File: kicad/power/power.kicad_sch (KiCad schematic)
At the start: 8 parts, among them J1 Power IN, J2 OLED_in, J3 SW_Power, J4 OLED_out, J5 Power OUT

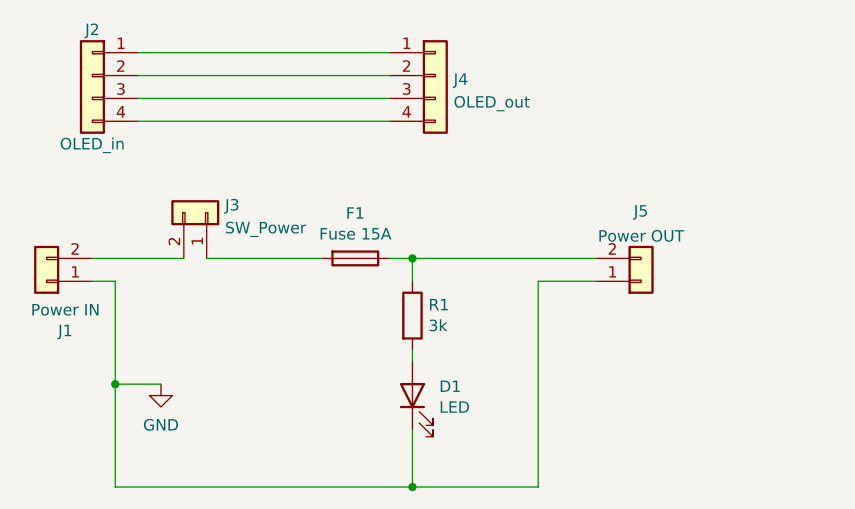
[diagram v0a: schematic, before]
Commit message: fix
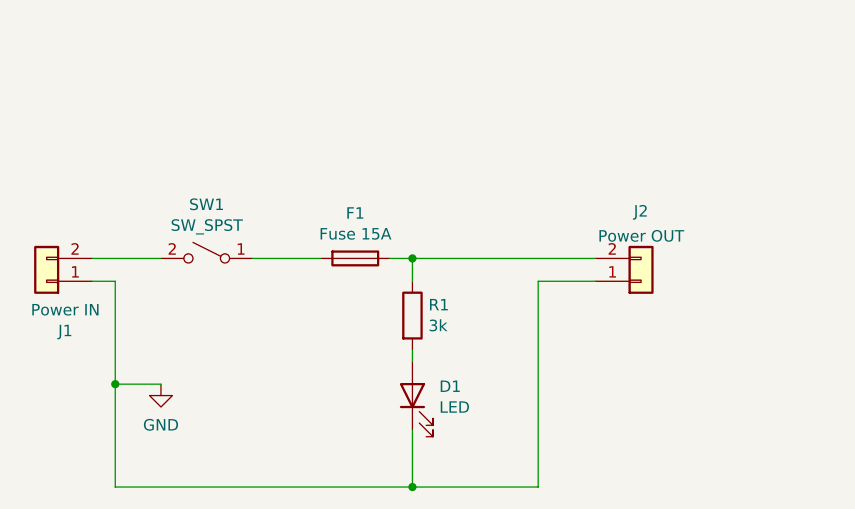
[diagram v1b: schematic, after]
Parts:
- removed J2: OLED_in, 0.main.robot:JSTS4B-ZRLFSN, symbol Connector_Generic:Conn_01x04
- removed J3: SW_Power, Connector_JST:JST_VH_B2PS-VH_1x02_P3.96mm_Horizontal, symbol Connector_Generic:Conn_01x02
- removed J4: OLED_out, Connector_PinSocket_2.54mm:PinSocket_1x04_P2.54mm_Vertical, symbol Connector_Generic:Conn_01x04
- added SW1: SW_SPST, 0.main.robot:SW_SPST_POWER, symbol Switch:SW_SPST
- renumbered J5 to J2
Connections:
- net at F1.2: now also SW1.1 (A)
- net at J1.2 (Pin_2): now also SW1.2 (B)
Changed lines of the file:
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@@
   (junction (at 162.56 83.82) (diameter 0) (color 0 0 0 0)
   )
-  (wire (pts (xy 162.56 83.82) (xy 162.56 86.36))
+  (wire (pts (xy 144.78 83.82) (xy 152.4 83.82))
     (stroke (width 0) (type default) (color 0 0 0 0))
   )
-  (wire (pts (xy 139.7 83.82) (xy 152.4 83.82))
+  (wire (pts (xy 162.56 83.82) (xy 162.56 86.36))
     (stroke (width 0) (type default) (color 0 0 0 0))
   )
@@
     (stroke (width 0) (type default) (color 0 0 0 0))
   )
-  (wire (pts (xy 127 83.82) (xy 137.16 83.82))
-    (stroke (width 0) (type default) (color 0 0 0 0))
-  )
   (wire (pts (xy 162.56 109.22) (xy 176.53 109.22))
     (stroke (width 0) (type default) (color 0 0 0 0))
   )
-  (wire (pts (xy 132.08 68.58) (xy 160.02 68.58))
+  (wire (pts (xy 127 86.36) (xy 129.54 86.36))
     (stroke (width 0) (type default) (color 0 0 0 0))
   )
-  (wire (pts (xy 127 86.36) (xy 129.54 86.36))
+  (wire (pts (xy 127 83.82) (xy 134.62 83.82))
     (stroke (width 0) (type default) (color 0 0 0 0))
   )
@@
     (stroke (width 0) (type default) (color 0 0 0 0))
   )
-  (wire (pts (xy 132.08 66.04) (xy 160.02 66.04))
-    (stroke (width 0) (type default) (color 0 0 0 0))
-  )
   (wire (pts (xy 162.56 83.82) (xy 182.88 83.82))
     (stroke (width 0) (type default) (color 0 0 0 0))
@@
     (stroke (width 0) (type default) (color 0 0 0 0))
   )
-  (wire (pts (xy 132.08 63.5) (xy 160.02 63.5))
-    (stroke (width 0) (type default) (color 0 0 0 0))
-  )
   (wire (pts (xy 176.53 86.36) (xy 182.88 86.36))
-    (stroke (width 0) (type default) (color 0 0 0 0))
-  )
-  (wire (pts (xy 132.08 60.96) (xy 160.02 60.96))
     (stroke (width 0) (type default) (color 0 0 0 0))
   )
@@
     (pin "2")
   )
-  (symbol (lib_id "Connector_Generic:Conn_01x04") (at 165.1 63.5 0) (unit 1)
-    (in_bom yes) (on_board yes) (fields_autoplaced)
-    (property "Reference" "J4" (id 0) (at 167.132 63.9353 0)
-      (effects (font (size 1.27 1.27)) (justify left))
-    )
-    (property "Value" "OLED_out" (id 1) (at 167.132 66.4722 0)
-      (effects (font (size 1.27 1.27)) (justify left))
-    )
-    (property "Footprint" "Connector_PinSocket_2.54mm:PinSocket_1x04_P2.54mm_Vertical" (id 2) (at 165.1 63.5 0)
-      (effects (font (size 1.27 1.27)) hide)
-    )
-    (property "Datasheet" "~" (id 3) (at 165.1 63.5 0)
-      (effects (font (size 1.27 1.27)) hide)
-    )
-    (pin "1")
-    (pin "2")
-    (pin "3")
-    (pin "4")
-  )
   (symbol (lib_id "Device:Fuse") (at 156.21 83.82 270) (unit 1)
     (in_bom yes) (on_board yes)
@@
     (pin "1")
     (pin "2")
-  )
-  (symbol (lib_id "Connector_Generic:Conn_01x02") (at 139.7 78.74 270) (mirror x) (unit 1)
-    (in_bom yes) (on_board yes) (fields_autoplaced)
-    (property "Reference" "J3" (id 0) (at 141.732 77.9053 90)
-      (effects (font (size 1.27 1.27)) (justify left))
-    )
-    (property "Value" "SW_Power" (id 1) (at 141.732 80.4422 90)
-      (effects (font (size 1.27 1.27)) (justify left))
-    )
-    (property "Footprint" "Connector_JST:JST_VH_B2PS-VH_1x02_P3.96mm_Horizontal" (id 2) (at 139.7 78.74 0)
-      (effects (font (size 1.27 1.27)) hide)
-    )
-    (property "Datasheet" "~" (id 3) (at 139.7 78.74 0)
-      (effects (font (size 1.27 1.27)) hide)
-    )
-    (pin "1")
-    (pin "2")
-  )
-  (symbol (lib_id "Connector_Generic:Conn_01x04") (at 127 63.5 0) (mirror y) (unit 1)
-    (in_bom yes) (on_board yes)
-    (property "Reference" "J2" (id 0) (at 127 58.42 0))
-    (property "Value" "OLED_in" (id 1) (at 127 71.12 0))
-    (property "Footprint" "0.main.robot:JSTS4B-ZRLFSN" (id 2) (at 127 63.5 0)
-      (effects (font (size 1.27 1.27)) hide)
-    )
-    (property "Datasheet" "~" (id 3) (at 127 63.5 0)
-      (effects (font (size 1.27 1.27)) hide)
-    )
-    (pin "1")
-    (pin "2")
-    (pin "3")
-    (pin "4")
   )
   (symbol (lib_id "Connector_Generic:Conn_01x02") (at 121.92 86.36 180) (unit 1)
@@
     (pin "2")
   )
+  (symbol (lib_id "Switch:SW_SPST") (at 139.7 83.82 0) (mirror y) (unit 1)
+    (in_bom yes) (on_board yes)
+    (property "Reference" "SW1" (id 0) (at 139.7 77.851 0))
+    (property "Value" "SW_SPST" (id 1) (at 139.7 80.1624 0))
+    (property "Footprint" "0.main.robot:SW_SPST_POWER" (id 2) (at 139.7 83.82 0)
+      (effects (font (size 1.27 1.27)) hide)
+    )
+    (property "Datasheet" "~" (id 3) (at 139.7 83.82 0)
+      (effects (font (size 1.27 1.27)) hide)
+    )
+    (pin "1")
+    (pin "2")
+  )
   (symbol (lib_id "Connector_Generic:Conn_01x02") (at 187.96 86.36 0) (mirror x) (unit 1)
     (in_bom yes) (on_board yes) (fields_autoplaced)
-    (property "Reference" "J5" (id 0) (at 187.96 78.5835 0))
+    (property "Reference" "J2" (id 0) (at 187.96 78.5835 0))
     (property "Value" "Power OUT" (id 1) (at 187.96 81.3586 0))
     (property "Footprint" "Connector_JST:JST_VH_B2PS-VH_1x02_P3.96mm_Horizontal" (id 2) (at 187.96 86.36 0)
@@
       (reference "J1") (unit 1) (value "Power IN") (footprint "0.main.robot:AMASS_XT60-M_1x02_P7.20mm_Vertical")
     )
-    (path "/598e9a76-0db2-44a9-a60c-d4ed24c476ce"
-      (reference "J2") (unit 1) (value "OLED_in") (footprint "0.main.robot:JSTS4B-ZRLFSN")
-    )
-    (path "/5499bae8-d48d-4f07-8f5a-e4889474cbb5"
-      (reference "J3") (unit 1) (value "SW_Power") (footprint "Connector_JST:JST_VH_B2PS-VH_1x02_P3.96mm_Horizontal")
-    )
-    (path "/10f6edf7-7273-449a-9f23-cf75ddf38fd1"
-      (reference "J4") (unit 1) (value "OLED_out") (footprint "Connector_PinSocket_2.54mm:PinSocket_1x04_P2.54mm_Vertical")
-    )
     (path "/885e45ca-60a4-45d9-b880-170c39d96ea5"
-      (reference "J5") (unit 1) (value "Power OUT") (footprint "Connector_JST:JST_VH_B2PS-VH_1x02_P3.96mm_Horizontal")
+      (reference "J2") (unit 1) (value "Power OUT") (footprint "Connector_JST:JST_VH_B2PS-VH_1x02_P3.96mm_Horizontal")
     )
     (path "/10672f86-6d1c-4735-823d-6815512456a3"
       (reference "R1") (unit 1) (value "3k") (footprint "Resistor_SMD:R_0603_1608Metric_Pad0.98x0.95mm_HandSolder")
     )
+    (path "/860b1473-4398-44af-9a5d-d556293557fc"
+      (reference "SW1") (unit 1) (value "SW_SPST") (footprint "0.main.robot:SW_SPST_POWER")
+    )
   )

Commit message: fix: power
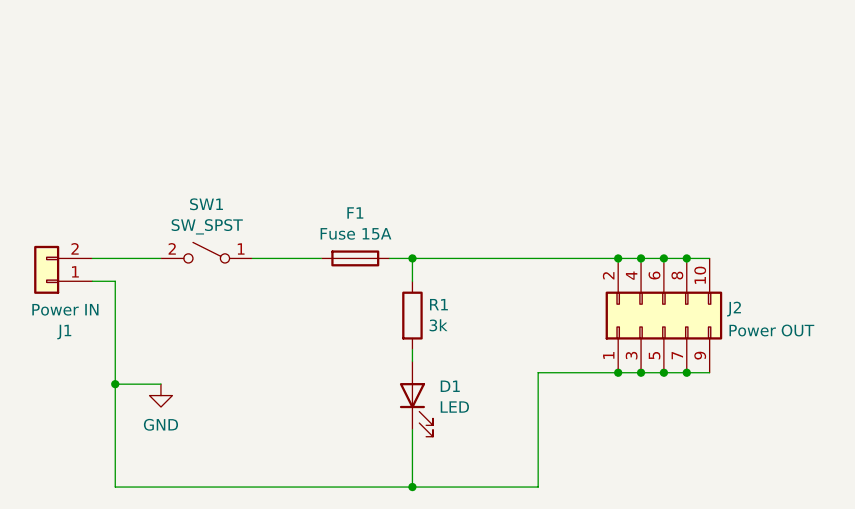
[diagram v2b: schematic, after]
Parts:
- removed J2: Power OUT, Connector_JST:JST_VH_B2PS-VH_1x02_P3.96mm_Horizontal, symbol Connector_Generic:Conn_01x02
- added J2: Power OUT, Connector_PinHeader_2.54mm:PinHeader_2x05_P2.54mm_Vertical, symbol Connector_Generic:Conn_02x05_Odd_Even
- F1: footprint 0.main.robot:FUSE_20mm -> 0.main.robot:FUSE_35222
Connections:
- net GND: now also J2.1 (Pin_1), J2.3 (Pin_3), J2.5 (Pin_5), J2.7 (Pin_7), J2.9 (Pin_9)
- net at F1.1, R1.1: now also J2.10 (Pin_10), J2.2 (Pin_2), J2.4 (Pin_4), J2.6 (Pin_6), J2.8 (Pin_8)
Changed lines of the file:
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@@
 (kicad_sch (version 20211123) (generator eeschema)
   (paper "A4")
+  (junction (at 193.04 96.52) (diameter 0) (color 0 0 0 0)
+  )
   (junction (at 162.56 109.22) (diameter 0) (color 0 0 0 0)
   )
   (junction (at 129.54 97.79) (diameter 0) (color 0 0 0 0)
   )
+  (junction (at 190.5 96.52) (diameter 0) (color 0 0 0 0)
+  )
+  (junction (at 190.5 83.82) (diameter 0) (color 0 0 0 0)
+  )
+  (junction (at 185.42 96.52) (diameter 0) (color 0 0 0 0)
+  )
+  (junction (at 187.96 83.82) (diameter 0) (color 0 0 0 0)
+  )
+  (junction (at 187.96 96.52) (diameter 0) (color 0 0 0 0)
+  )
+  (junction (at 185.42 83.82) (diameter 0) (color 0 0 0 0)
+  )
   (junction (at 162.56 83.82) (diameter 0) (color 0 0 0 0)
   )
+  (junction (at 193.04 83.82) (diameter 0) (color 0 0 0 0)
+  )
   (wire (pts (xy 144.78 83.82) (xy 152.4 83.82))
     (stroke (width 0) (type default) (color 0 0 0 0))
@@
     (stroke (width 0) (type default) (color 0 0 0 0))
   )
+  (wire (pts (xy 190.5 83.82) (xy 193.04 83.82))
+    (stroke (width 0) (type default) (color 0 0 0 0))
+  )
   (wire (pts (xy 127 86.36) (xy 129.54 86.36))
     (stroke (width 0) (type default) (color 0 0 0 0))
   )
+  (wire (pts (xy 193.04 83.82) (xy 195.58 83.82))
+    (stroke (width 0) (type default) (color 0 0 0 0))
+  )
   (wire (pts (xy 127 83.82) (xy 134.62 83.82))
     (stroke (width 0) (type default) (color 0 0 0 0))
@@
     (stroke (width 0) (type default) (color 0 0 0 0))
   )
-  (wire (pts (xy 176.53 109.22) (xy 176.53 86.36))
+  (wire (pts (xy 176.53 109.22) (xy 176.53 96.52))
+    (stroke (width 0) (type default) (color 0 0 0 0))
+  )
+  (wire (pts (xy 185.42 96.52) (xy 187.96 96.52))
+    (stroke (width 0) (type default) (color 0 0 0 0))
+  )
+  (wire (pts (xy 187.96 96.52) (xy 190.5 96.52))
     (stroke (width 0) (type default) (color 0 0 0 0))
   )
@@
     (stroke (width 0) (type default) (color 0 0 0 0))
   )
-  (wire (pts (xy 162.56 83.82) (xy 182.88 83.82))
+  (wire (pts (xy 162.56 83.82) (xy 185.42 83.82))
     (stroke (width 0) (type default) (color 0 0 0 0))
   )
@@
     (stroke (width 0) (type default) (color 0 0 0 0))
   )
-  (wire (pts (xy 176.53 86.36) (xy 182.88 86.36))
+  (wire (pts (xy 185.42 83.82) (xy 187.96 83.82))
+    (stroke (width 0) (type default) (color 0 0 0 0))
+  )
+  (wire (pts (xy 176.53 96.52) (xy 185.42 96.52))
+    (stroke (width 0) (type default) (color 0 0 0 0))
+  )
+  (wire (pts (xy 193.04 96.52) (xy 195.58 96.52))
+    (stroke (width 0) (type default) (color 0 0 0 0))
+  )
+  (wire (pts (xy 190.5 96.52) (xy 193.04 96.52))
     (stroke (width 0) (type default) (color 0 0 0 0))
   )
   (wire (pts (xy 129.54 97.79) (xy 134.62 97.79))
+    (stroke (width 0) (type default) (color 0 0 0 0))
+  )
+  (wire (pts (xy 187.96 83.82) (xy 190.5 83.82))
     (stroke (width 0) (type default) (color 0 0 0 0))
   )
@@
     (property "Reference" "F1" (id 0) (at 156.21 78.8162 90))
     (property "Value" "Fuse 15A" (id 1) (at 156.21 81.1276 90))
-    (property "Footprint" "0.main.robot:FUSE_20mm" (id 2) (at 156.21 82.042 90)
+    (property "Footprint" "0.main.robot:FUSE_35222" (id 2) (at 156.21 82.042 90)
       (effects (font (size 1.27 1.27)) hide)
     )
@@
     (pin "2")
   )
+  (symbol (lib_id "Connector_Generic:Conn_02x05_Odd_Even") (at 190.5 91.44 90) (unit 1)
+    (in_bom yes) (on_board yes) (fields_autoplaced)
+    (property "Reference" "J2" (id 0) (at 197.612 89.3353 90)
+      (effects (font (size 1.27 1.27)) (justify right))
+    )
+    (property "Value" "Power OUT" (id 1) (at 197.612 91.8722 90)
+      (effects (font (size 1.27 1.27)) (justify right))
+    )
+    (property "Footprint" "Connector_PinHeader_2.54mm:PinHeader_2x05_P2.54mm_Vertical" (id 2) (at 190.5 91.44 0)
+      (effects (font (size 1.27 1.27)) hide)
+    )
+    (property "Datasheet" "~" (id 3) (at 190.5 91.44 0)
+      (effects (font (size 1.27 1.27)) hide)
+    )
+    (pin "1")
+    (pin "10")
+    (pin "2")
+    (pin "3")
+    (pin "4")
+    (pin "5")
+    (pin "6")
+    (pin "7")
+    (pin "8")
+    (pin "9")
+  )
   (symbol (lib_id "Switch:SW_SPST") (at 139.7 83.82 0) (mirror y) (unit 1)
     (in_bom yes) (on_board yes)
@@
     (pin "2")
   )
-  (symbol (lib_id "Connector_Generic:Conn_01x02") (at 187.96 86.36 0) (mirror x) (unit 1)
-    (in_bom yes) (on_board yes) (fields_autoplaced)
-    (property "Reference" "J2" (id 0) (at 187.96 78.5835 0))
-    (property "Value" "Power OUT" (id 1) (at 187.96 81.3586 0))
-    (property "Footprint" "Connector_JST:JST_VH_B2PS-VH_1x02_P3.96mm_Horizontal" (id 2) (at 187.96 86.36 0)
-      (effects (font (size 1.27 1.27)) hide)
-    )
-    (property "Datasheet" "~" (id 3) (at 187.96 86.36 0)
-      (effects (font (size 1.27 1.27)) hide)
-    )
-    (pin "1")
-    (pin "2")
-  )
   (symbol (lib_id "power:GND") (at 134.62 97.79 0) (unit 1)
     (in_bom yes) (on_board yes) (fields_autoplaced)
@@
     )
     (path "/26c79640-a484-4e7e-adea-f221c3f9ae2e"
-      (reference "F1") (unit 1) (value "Fuse 15A") (footprint "0.main.robot:FUSE_20mm")
+      (reference "F1") (unit 1) (value "Fuse 15A") (footprint "0.main.robot:FUSE_35222")
     )
     (path "/627fc830-2e08-4594-9783-a727f28edeaa"
       (reference "J1") (unit 1) (value "Power IN") (footprint "0.main.robot:AMASS_XT60-M_1x02_P7.20mm_Vertical")
     )
-    (path "/885e45ca-60a4-45d9-b880-170c39d96ea5"
-      (reference "J2") (unit 1) (value "Power OUT") (footprint "Connector_JST:JST_VH_B2PS-VH_1x02_P3.96mm_Horizontal")
+    (path "/81c9dfc0-c050-42fd-a83d-7eb9ee4bba76"
+      (reference "J2") (unit 1) (value "Power OUT") (footprint "Connector_PinHeader_2.54mm:PinHeader_2x05_P2.54mm_Vertical")
     )
     (path "/10672f86-6d1c-4735-823d-6815512456a3"
